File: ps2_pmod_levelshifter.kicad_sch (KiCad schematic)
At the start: 4 parts, among them J1 PS/2, J2 PMOD, J3 EXT_POWER

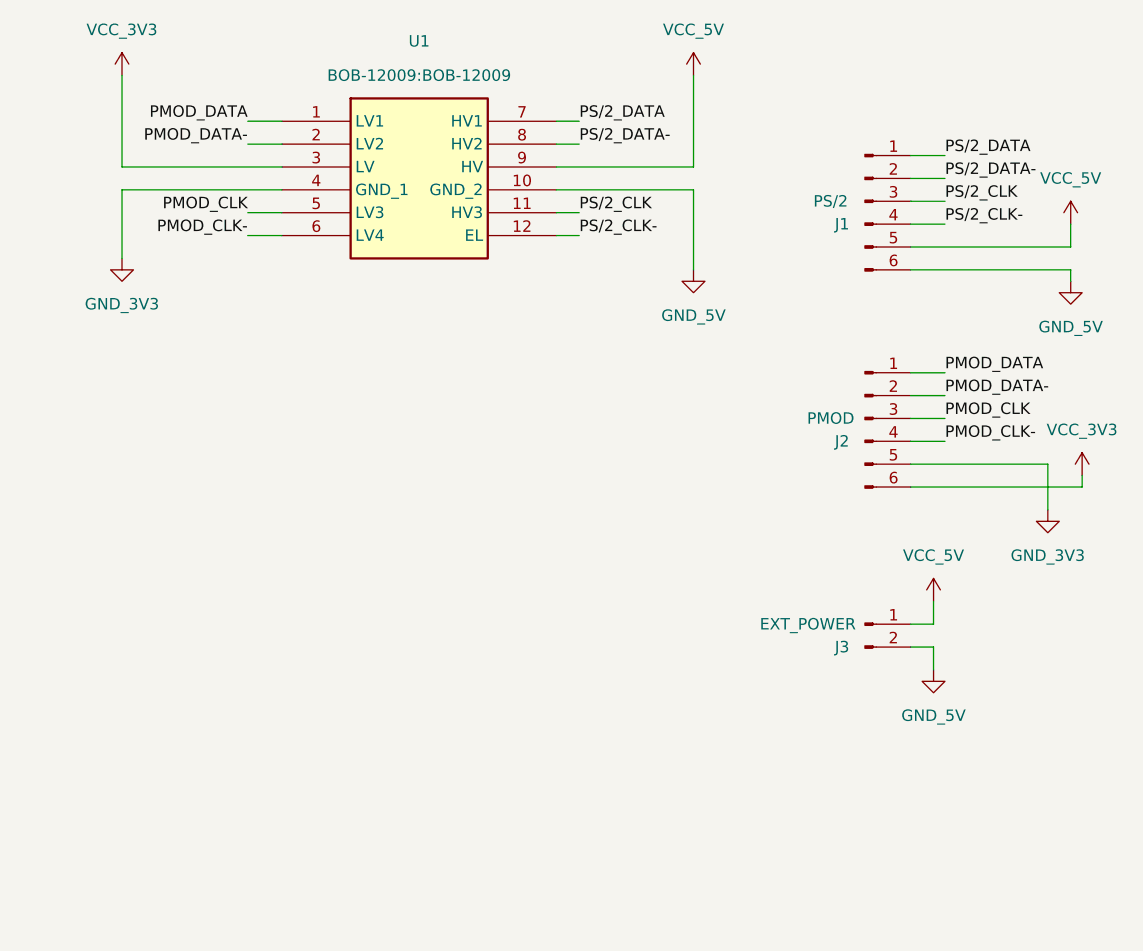
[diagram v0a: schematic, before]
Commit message: update design
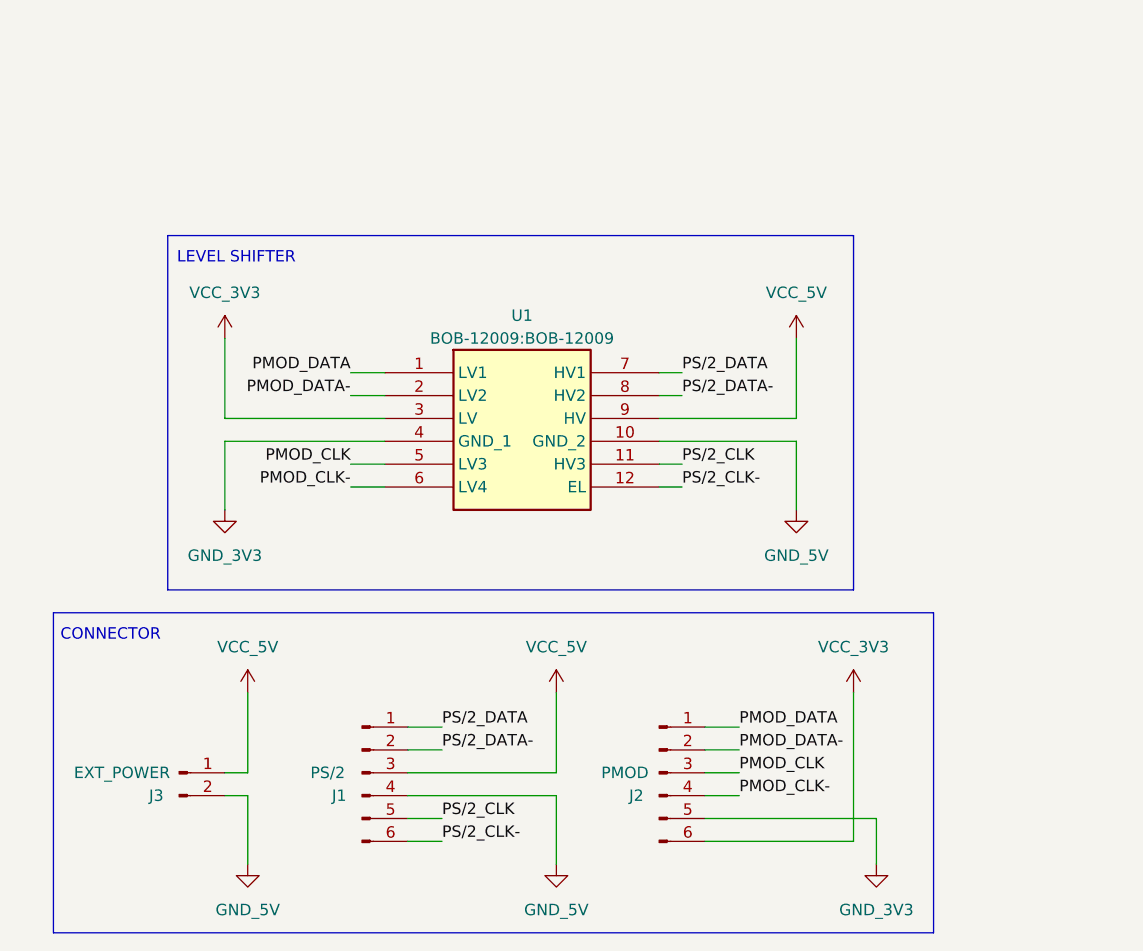
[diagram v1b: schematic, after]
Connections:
- net GND_5V: now also J1.4 (Pin_4); no longer J1.6 (Pin_6)
- net PS/2_CLK: now also J1.5 (Pin_5); no longer J1.3 (Pin_3)
- net PS/2_CLK-: now also J1.6 (Pin_6); no longer J1.4 (Pin_4)
- net VCC_5V: now also J1.3 (Pin_3); no longer J1.5 (Pin_5)
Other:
- note added: "CONNECTOR"
- note added: "LEVEL SHIFTER"
- moved on the sheet: J1, J2, J3, U1

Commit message: update design
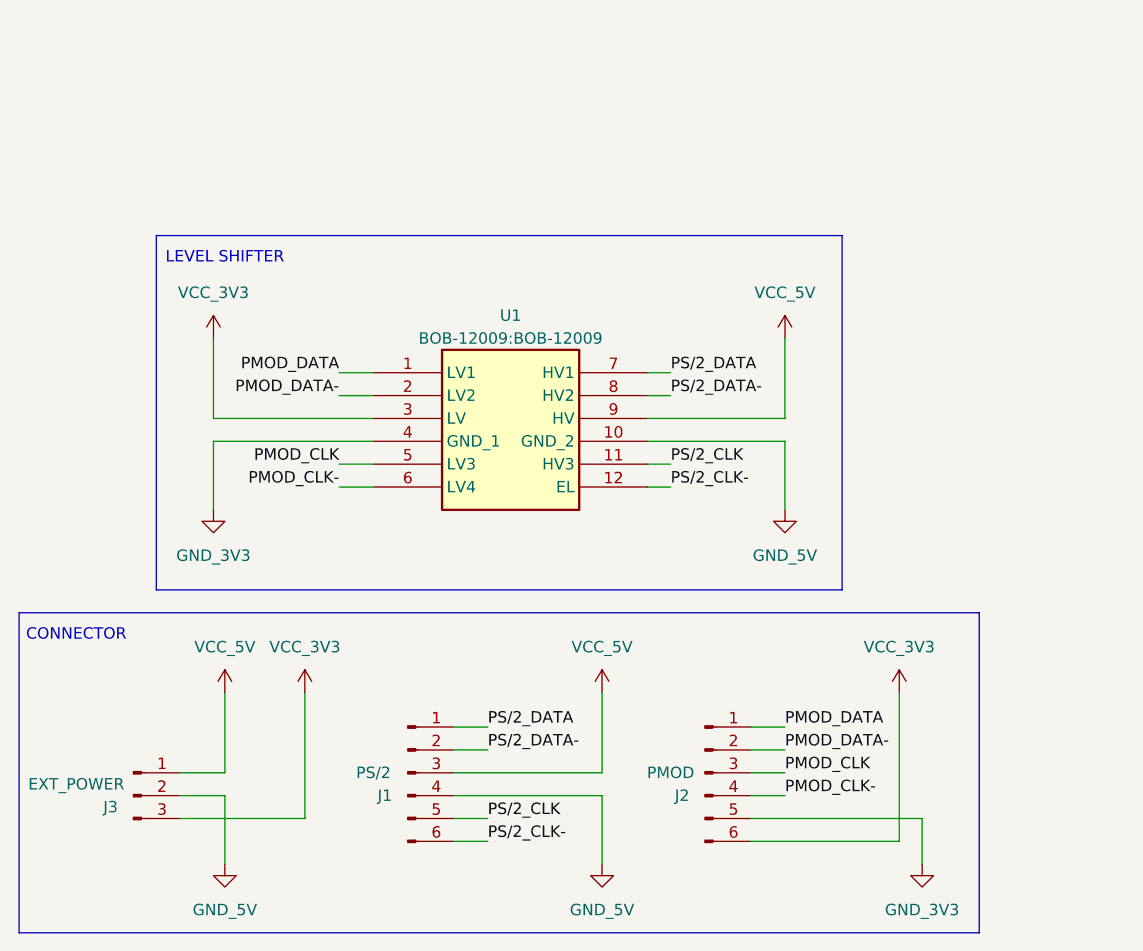
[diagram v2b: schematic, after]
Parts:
- removed J3: EXT_POWER, Connector_PinHeader_2.54mm:PinHeader_1x02_P2.54mm_Vertical, symbol Connector:Conn_01x02_Pin
- added J3: EXT_POWER, Connector_PinHeader_2.54mm:PinHeader_1x03_P2.54mm_Vertical, symbol Connector:Conn_01x03_Pin
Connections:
- net GND_5V: now also J3.2 (Pin_2)
- net VCC_3V3: now also J3.3 (Pin_3)
- net VCC_5V: now also J3.1 (Pin_1)
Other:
- moved on the sheet: J1, J2, U1

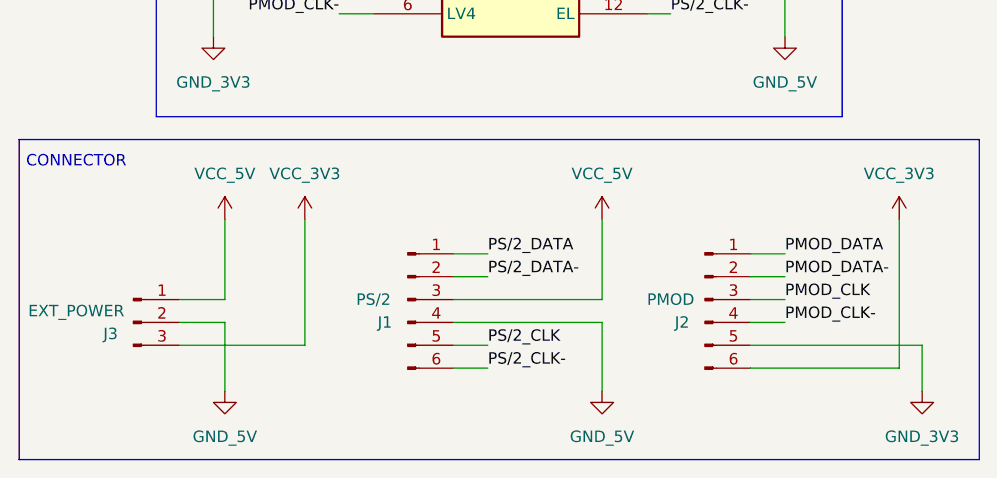
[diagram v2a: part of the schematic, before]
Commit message: update design
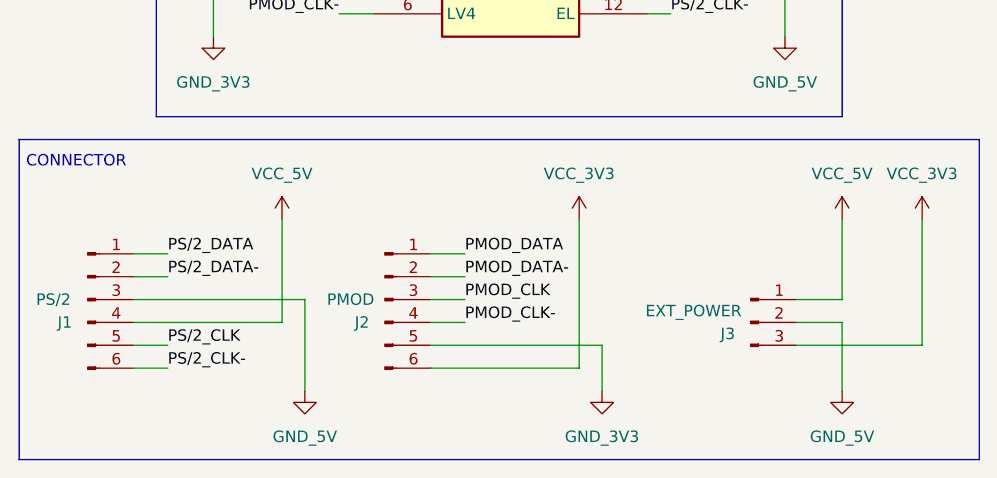
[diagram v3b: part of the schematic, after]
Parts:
- J1: footprint r_mini_din:Mini_din6 -> ps2-connector:ps2_mini_din6
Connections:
- net GND_5V: now also J1.3 (Pin_3); no longer J1.4 (Pin_4)
- net VCC_5V: now also J1.4 (Pin_4); no longer J1.3 (Pin_3)
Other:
- moved on the sheet: J1, J2, J3
